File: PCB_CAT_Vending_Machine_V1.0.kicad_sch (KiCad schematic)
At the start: 4 parts

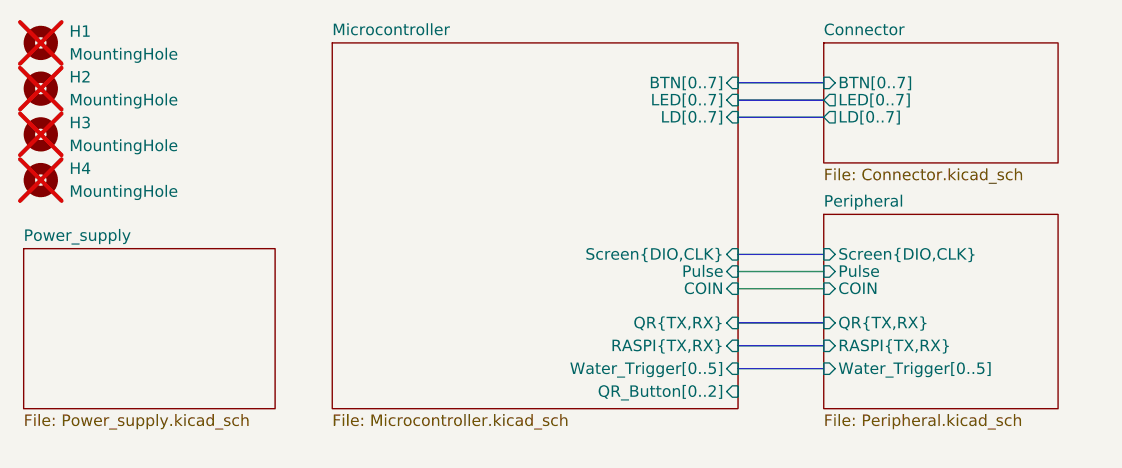
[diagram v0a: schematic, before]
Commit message: finish no review
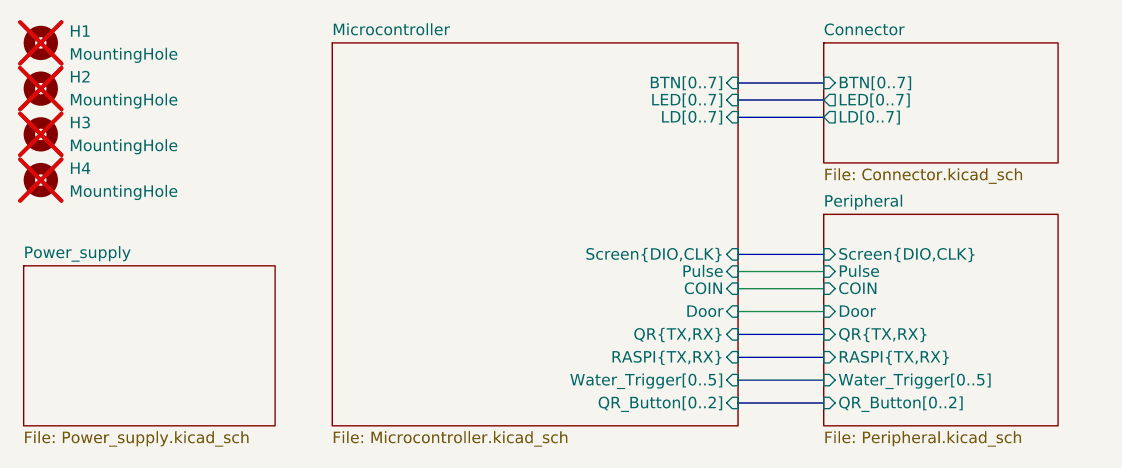
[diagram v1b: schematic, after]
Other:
- sheet Microcontroller ports: added Door; removed none
- sheet Peripheral ports: added Door, QR_Button[0..2]; removed none
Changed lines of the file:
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@@
 	(bus
 		(pts
-			(xy 168.91 104.14) (xy 178.435 104.14)
+			(xy 168.91 105.41) (xy 178.435 105.41)
 		)
 		(stroke
@@
 	(bus
 		(pts
-			(xy 168.91 106.68) (xy 178.435 106.68)
+			(xy 168.91 107.95) (xy 178.435 107.95)
+		)
+		(stroke
+			(width 0)
+			(type default)
+		)
+	)
+	(bus
+		(pts
+			(xy 168.91 110.49) (xy 178.435 110.49)
 		)
 		(stroke
@@
 	(bus
 		(pts
-			(xy 168.91 101.6) (xy 178.435 101.6)
+			(xy 168.91 102.87) (xy 178.435 102.87)
 		)
 		(stroke
@@
 		(pts
 			(xy 168.91 93.98) (xy 178.435 93.98)
+		)
+		(stroke
+			(width 0)
+			(type default)
+		)
+	)
+	(wire
+		(pts
+			(xy 168.91 100.33) (xy 178.435 100.33)
 		)
 		(stroke
@@
 	(sheet
 		(at 178.435 89.535)
-		(size 26.035 21.59)
+		(size 26.035 23.495)
 		(exclude_from_sim no)
 		(in_bom yes)
@@
 		)
 		(property "Sheetfile" "Peripheral.kicad_sch"
-			(at 178.435 111.7096 0)
+			(at 178.435 113.6146 0)
 			(effects
 				(font
@@
 		)
 		(pin "QR{TX,RX}" input
-			(at 178.435 101.6 180)
+			(at 178.435 102.87 180)
 			(effects
 				(font
@@
 		)
 		(pin "RASPI{TX,RX}" input
-			(at 178.435 104.14 180)
+			(at 178.435 105.41 180)
 			(effects
 				(font
@@
 		)
 		(pin "Water_Trigger[0..5]" input
-			(at 178.435 106.68 180)
+			(at 178.435 107.95 180)
+			(effects
+				(font
+					(size 1.27 1.27)
+				)
+				(justify left)
+			)
+		)
+		(pin "QR_Button[0..2]" input
+			(at 178.435 110.49 180)
+			(effects
+				(font
+					(size 1.27 1.27)
+				)
+				(justify left)
+			)
+		)
+		(pin "Door" input
+			(at 178.435 100.33 180)
 			(effects
 				(font
@@
 	)
 	(sheet
-		(at 89.535 93.345)
+		(at 89.535 95.25)
 		(size 27.94 17.78)
 		(exclude_from_sim no)
@@
 		)
 		(property "Sheetname" "Power_supply"
-			(at 89.535 92.6334 0)
+			(at 89.535 94.5384 0)
 			(effects
 				(font
@@
 		)
 		(property "Sheetfile" "Power_supply.kicad_sch"
-			(at 89.535 111.7096 0)
+			(at 89.535 113.6146 0)
 			(effects
 				(font
@@
 	(sheet
 		(at 123.825 70.485)
-		(size 45.085 40.64)
+		(size 45.085 42.545)
 		(exclude_from_sim no)
 		(in_bom yes)
@@
 		)
 		(property "Sheetfile" "Microcontroller.kicad_sch"
-			(at 123.825 111.7096 0)
+			(at 123.825 113.6146 0)
 			(effects
 				(font
@@
 		)
 		(pin "QR{TX,RX}" input
-			(at 168.91 101.6 0)
+			(at 168.91 102.87 0)
 			(effects
 				(font
@@
 		)
 		(pin "RASPI{TX,RX}" input
-			(at 168.91 104.14 0)
+			(at 168.91 105.41 0)
 			(effects
 				(font
@@
 		)
 		(pin "Water_Trigger[0..5]" input
-			(at 168.91 106.68 0)
+			(at 168.91 107.95 0)
 			(effects
 				(font
@@
 		)
 		(pin "QR_Button[0..2]" input
-			(at 168.91 109.22 0)
-			(effects
-				(font
+			(at 168.91 110.49 0)
+			(effects
+				(font
+					(size 1.27 1.27)
+				)
+				(justify right)
+			)
+		)
+		(pin "Door" input
+			(at 168.91 100.33 0)
+			(effects
+				(font
